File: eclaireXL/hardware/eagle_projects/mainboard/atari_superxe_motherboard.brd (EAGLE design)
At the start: 140.6 x 100.1 mm, 147 parts, among them U1 EPCS

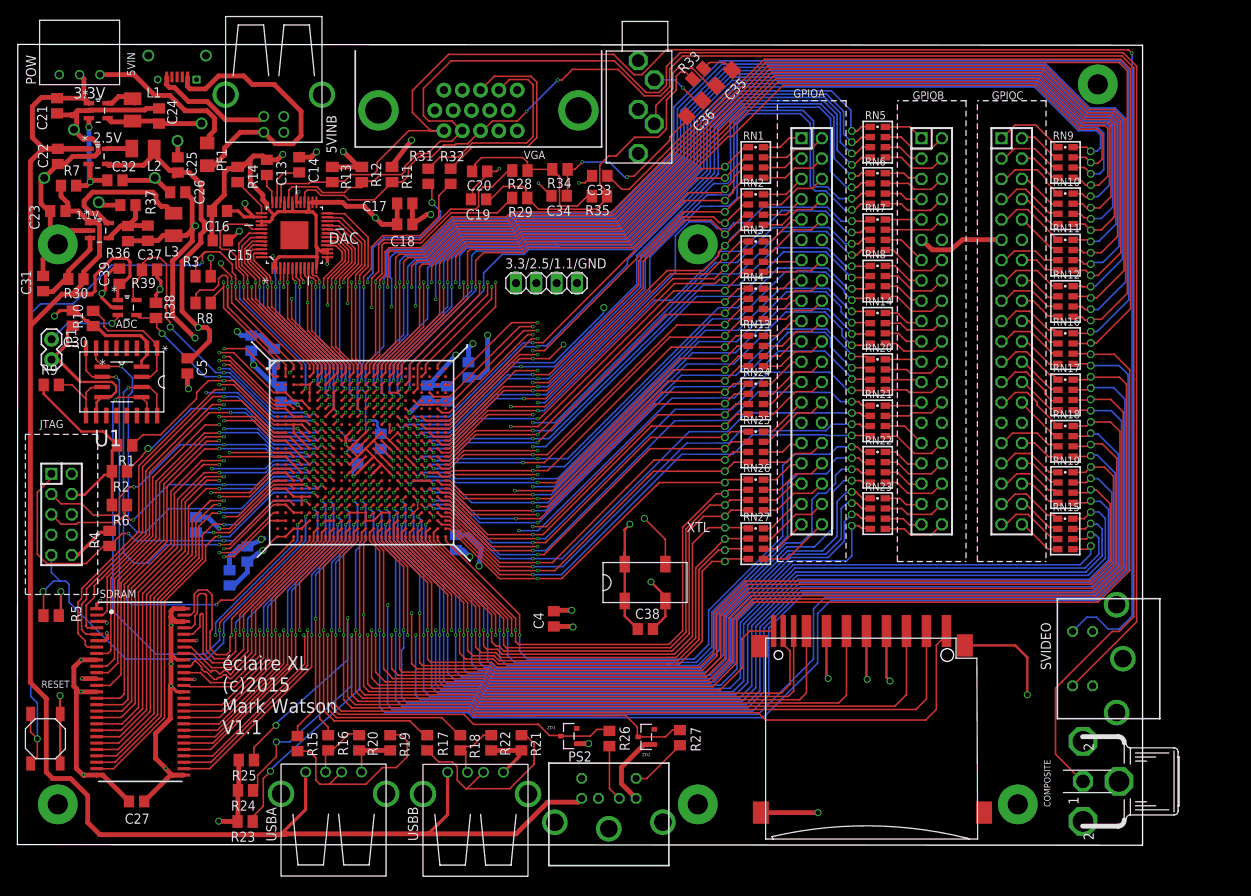
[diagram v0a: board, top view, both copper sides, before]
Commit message: DE1 connector spacing (20mm). Improved mounting holes.
git-svn-id: http://www.64kib.com/atarixlfpga_svn/trunk/atari_800xl@411 d6161ac3-aae1-4d52-9b05-ea9ac36b53d3
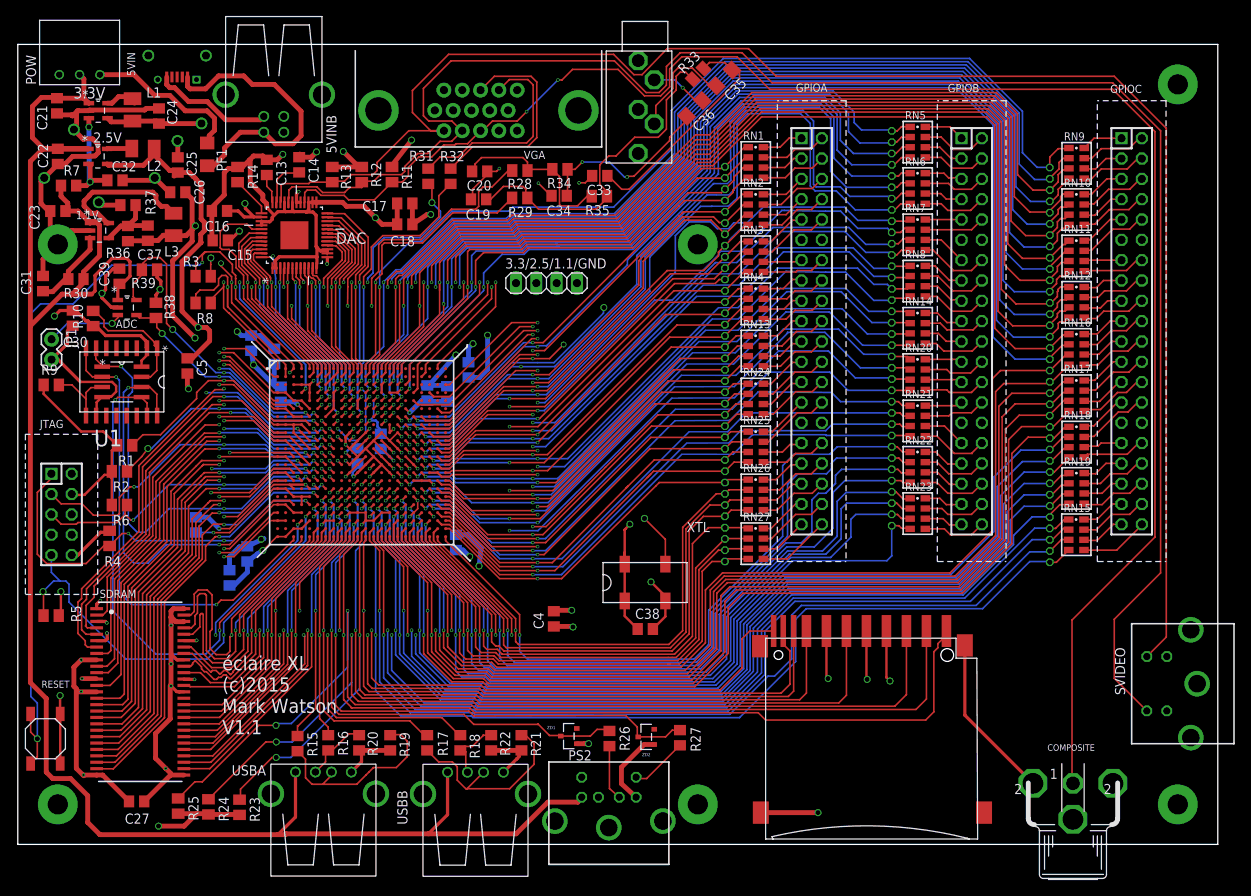
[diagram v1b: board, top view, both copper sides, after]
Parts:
- moved H6 20.0 mm to (145.0, 5.00)
- moved GPIOC 15.0 mm to (139.2, 64.1)
- moved R25 10.3 mm to (20.0, 4.79), turned to 270 degrees
- moved H1 10.0 mm to (145.0, 95.0)
- moved SVIDEO 9.79 mm to (152.1, 20.1)
- moved U$3 5.51 mm to (129.0, 59.2)
- moved R24 5.07 mm to (23.8, 4.69), turned to 270 degrees
- moved GPIOB 5.00 mm to (119.2, 64.1)
- moved RN14 5.00 mm to (112.5, 64.5)
- moved RN20 5.00 mm to (112.5, 58.7)
- moved RN21 5.00 mm to (112.5, 52.9)
- moved RN22 5.00 mm to (112.5, 47.1)
- moved RN23 5.00 mm to (112.5, 41.4)
- moved RN5 5.00 mm to (112.5, 87.8)
- moved RN6 5.00 mm to (112.5, 82.0)
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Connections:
- removed net N$134: GPIOC.40, RN15.4
- new net N$15: GPIOC.1, RN9.8
- net GPIOC0: now also RN9.1, U$1.B12; no longer RN9.8, U$1.C15
- net GPIOC1: now also RN9.2, U$1.D12; no longer RN9.7, U$1.E15
- net GPIOC10: now also RN11.3, U$1.A14; no longer RN11.6, U$1.C13
- net GPIOC11: now also RN11.4, U$1.E14; no longer RN11.5, U$1.D13
- net GPIOC12: now also RN12.1, U$1.F14; no longer RN12.8, U$1.B13
- net GPIOC13: now also RN12.2, U$1.H14; no longer RN12.7, U$1.A13
- net GPIOC14: now also RN12.3, U$1.A15; no longer RN12.6, U$1.F12
- net GPIOC15: now also RN12.4, U$1.B15; no longer RN12.5, U$1.E12
- net GPIOC16: now also RN16.1, U$1.E15; no longer RN16.8, U$1.D12
- net GPIOC17: now also RN16.2, U$1.C15; no longer RN16.7, U$1.B12
- net GPIOC18: now also RN16.3, U$1.Y16; no longer RN16.6, U$1.V13
- net GPIOC19: now also RN16.4, U$1.V16; no longer RN16.5, U$1.AA13
- net GPIOC2: now also RN9.3, U$1.E12; no longer RN9.6, U$1.B15
- net GPIOC20: now also RN17.1, U$1.W16; no longer RN17.8, U$1.AB13
- net GPIOC21: now also RN17.2, U$1.U16; no longer RN17.7, U$1.R14
- net GPIOC22: now also RN17.3, U$1.AB15; no longer RN17.6, U$1.T14
- net GPIOC23: now also RN17.4, U$1.AA15; no longer RN17.5, U$1.Y14
- net GPIOC24: now also RN18.1, U$1.V15; no longer RN18.8, U$1.V14
- net GPIOC25: now also RN18.2, U$1.Y15; no longer RN18.7, U$1.AA14
- net GPIOC26: now also RN18.3, U$1.U15; no longer RN18.6, U$1.T15
- net GPIOC27: now also RN18.4, U$1.T15; no longer RN18.5, U$1.U15
- net GPIOC28: now also RN19.1, U$1.AA14; no longer RN19.8, U$1.Y15
- net GPIOC29: now also RN19.2, U$1.V14; no longer RN19.7, U$1.V15
- net GPIOC3: now also RN9.4, U$1.F12; no longer RN9.5, U$1.A15
- net GPIOC30: now also RN19.3, U$1.Y14; no longer RN19.6, U$1.AA15
- net GPIOC31: now also RN19.4, U$1.T14; no longer RN19.5, U$1.AB15
- net GPIOC32: now also RN15.1, U$1.R14; no longer RN15.8, U$1.U16
- net GPIOC33: now also RN15.2, U$1.AB13; no longer RN15.7, U$1.W16
- net GPIOC34: now also RN15.3, U$1.AA13; no longer RN15.6, U$1.V16
- net GPIOC35: now also RN15.4, U$1.V13; no longer RN15.5, U$1.Y16
- net GPIOC4: now also RN10.1, U$1.A13; no longer RN10.8, U$1.H14
- net GPIOC5: now also RN10.2, U$1.B13; no longer RN10.7, U$1.F14
- net GPIOC6: now also RN10.3, U$1.D13; no longer RN10.6, U$1.E14
- net GPIOC7: now also RN10.4, U$1.C13; no longer RN10.5, U$1.A14
- net GPIOC8: now also RN11.1, U$1.F13; no longer RN11.8, U$1.G13
- net GPIOC9: now also RN11.2, U$1.G13; no longer RN11.7, U$1.F13
- net N$100: now also GPIOC.3, RN9.6; no longer GPIOC.2, RN9.2
- net N$101: now also GPIOC.4, RN9.5; no longer GPIOC.3, RN9.3
- net N$102: now also GPIOC.5, RN10.8; no longer GPIOC.4, RN9.4
- net N$103: now also GPIOC.6, RN10.7; no longer GPIOC.5, RN10.1
- net N$104: now also GPIOC.7, RN10.6; no longer GPIOC.6, RN10.2
- net N$105: now also GPIOC.8, RN10.5; no longer GPIOC.7, RN10.3
- net N$106: now also GPIOC.9, RN11.8; no longer GPIOC.8, RN10.4
- net N$107: now also GPIOC.10, RN11.7; no longer GPIOC.9, RN11.1
- net N$108: now also GPIOC.13, RN11.6; no longer GPIOC.10, RN11.2
- net N$109: now also GPIOC.14, RN11.5; no longer GPIOC.13, RN11.3
- net N$110: now also GPIOC.15, RN12.8; no longer GPIOC.14, RN11.4
- net N$111: now also GPIOC.16, RN12.7; no longer GPIOC.15, RN12.1
- net N$112: now also GPIOC.17, RN12.6; no longer GPIOC.16, RN12.2
- net N$113: now also GPIOC.18, RN12.5; no longer GPIOC.17, RN12.3
- net N$114: now also GPIOC.19, RN16.8; no longer GPIOC.18, RN12.4
- net N$115: now also GPIOC.20, RN16.7; no longer GPIOC.19, RN16.1
- net N$116: now also GPIOC.21, RN16.6; no longer GPIOC.20, RN16.2
- net N$117: now also GPIOC.22, RN16.5; no longer GPIOC.21, RN16.3
- net N$118: now also GPIOC.23, RN17.8; no longer GPIOC.22, RN16.4
- net N$119: now also GPIOC.24, RN17.7; no longer GPIOC.23, RN17.1
- net N$120: now also GPIOC.25, RN17.6; no longer GPIOC.24, RN17.2
- net N$121: now also GPIOC.26, RN17.5; no longer GPIOC.25, RN17.3
- net N$122: now also GPIOC.27, RN18.8; no longer GPIOC.26, RN17.4
- net N$123: now also GPIOC.28, RN18.7; no longer GPIOC.27, RN18.1
- net N$124: now also GPIOC.31, RN18.6; no longer GPIOC.28, RN18.2
- net N$125: now also GPIOC.32, RN18.5; no longer GPIOC.31, RN18.3
- net N$126: now also GPIOC.33, RN19.8; no longer GPIOC.32, RN18.4
- net N$127: now also GPIOC.34, RN19.7; no longer GPIOC.33, RN19.1
- net N$128: now also GPIOC.35, RN19.6; no longer GPIOC.34, RN19.2
- net N$129: now also GPIOC.36, RN19.5; no longer GPIOC.35, RN19.3
- net N$130: now also GPIOC.37, RN15.8; no longer GPIOC.36, RN19.4
- net N$131: now also GPIOC.38, RN15.7; no longer GPIOC.37, RN15.1
- net N$132: now also GPIOC.39, RN15.6; no longer GPIOC.38, RN15.2
- net N$133: now also GPIOC.40, RN15.5; no longer GPIOC.39, RN15.3
- net N$99: now also GPIOC.2, RN9.7; no longer GPIOC.1, RN9.1
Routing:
- net GPIOC21: track 160.9 -> 130.1 mm
- net GPIOC18: track 158.7 -> 128.7 mm, vias 2 -> 1
- net GPIOC19: track 160.2 -> 130.4 mm, vias 1 -> 2
- net GPIOC16: track 163.0 -> 133.7 mm
- net GPIOC14: track 157.4 -> 129.4 mm, vias 2 -> 1
- net GPIOC23: track 152.0 -> 125.0 mm, vias 2 -> 1
- net GPIOC22: track 150.8 -> 124.6 mm, vias 2 -> 1
- net GPIOC25: track 145.7 -> 121.3 mm, vias 1 -> 2
- net GPIOC15: track 159.0 -> 136.6 mm, vias 2 -> 1
- net 5V0: track 408.9 -> 431.0 mm
- net GPIOC20: track 150.0 -> 128.5 mm, vias 1 -> 2
- net GPIOC17: track 159.2 -> 138.7 mm, vias 1 -> 2
- net GPIOC27: track 144.1 -> 125.0 mm
- net GPIOC10: track 143.9 -> 124.9 mm, vias 2 -> 1
- net SD_CS: track 132.9 -> 151.3 mm
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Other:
- board size 140.6 x 100.1 mm -> 150 x 100 mm
